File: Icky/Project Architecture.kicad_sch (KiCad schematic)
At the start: 8 parts

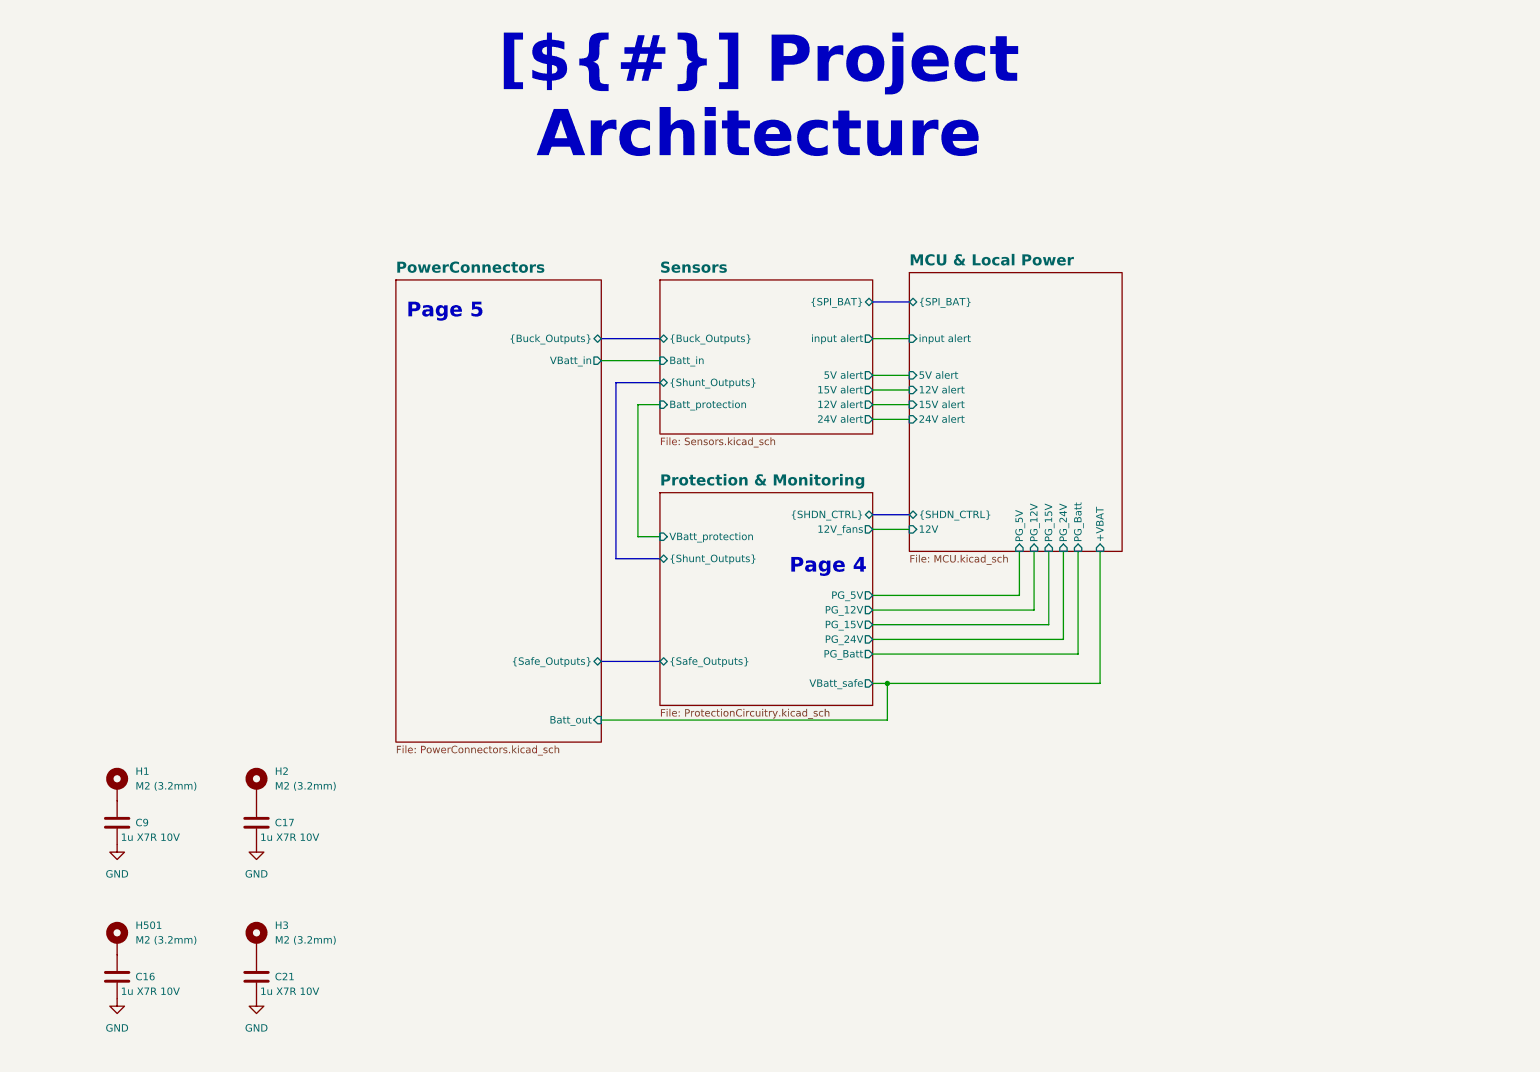
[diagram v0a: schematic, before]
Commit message: ERC passed
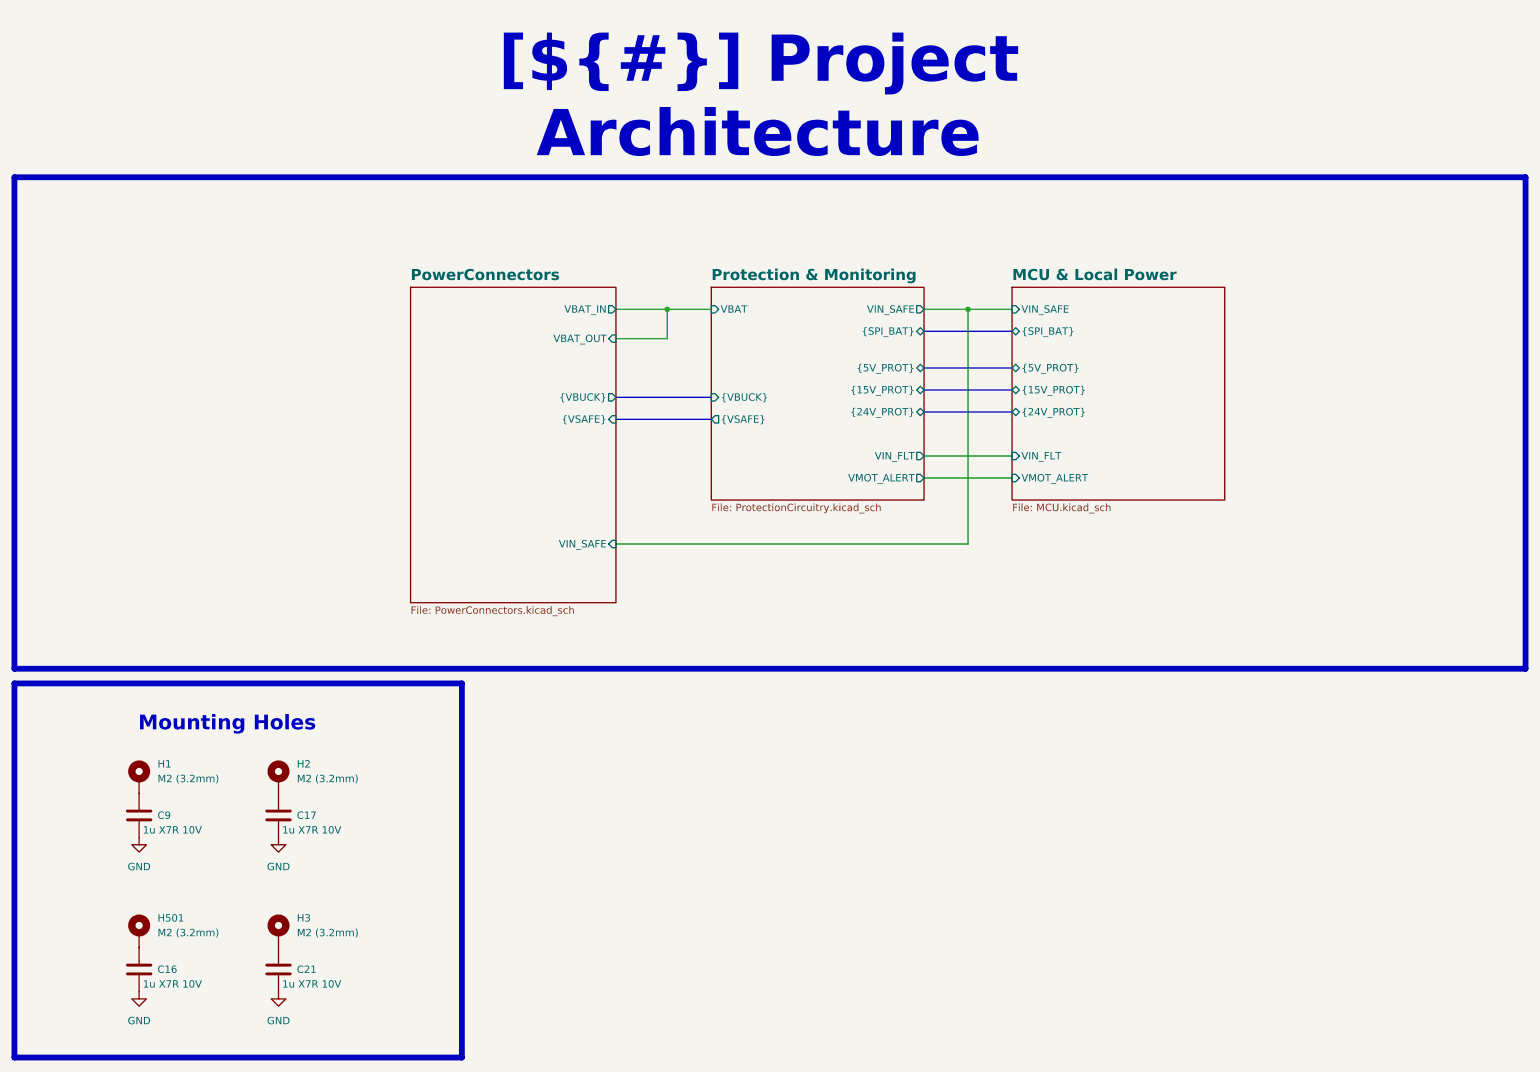
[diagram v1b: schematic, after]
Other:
- removed sheet Sensors
- sheet MCU & Local Power ports: added VIN_FLT, VIN_SAFE, VMOT_ALERT, {15V_PROT}, {24V_PROT}, {5V_PROT}; removed +VBAT, 12V, 12V alert, 15V alert, 24V alert, 5V alert, PG_12V, PG_15V, PG_24V, PG_5V, PG_Batt, input alert, {SHDN_CTRL}
- sheet PowerConnectors ports: added VBAT_IN, VBAT_OUT, VIN_SAFE, {VBUCK}, {VSAFE}; removed Batt_out, VBatt_in, {Buck_Outputs}, {Safe_Outputs}
- sheet Protection & Monitoring ports: added VBAT, VIN_FLT, VIN_SAFE, VMOT_ALERT, {15V_PROT}, {24V_PROT}, {5V_PROT}, {SPI_BAT}, {VBUCK}, {VSAFE}; removed 12V_fans, PG_12V, PG_15V, PG_24V, PG_5V, PG_Batt, VBatt_protection, VBatt_safe, {SHDN_CTRL}, {Safe_Outputs}, {Shunt_Outputs}
- note removed: "Page 4"
- note removed: "Page 5"
- moved on the sheet: C16, C17, C21, C9, H1, H2, H3, H501

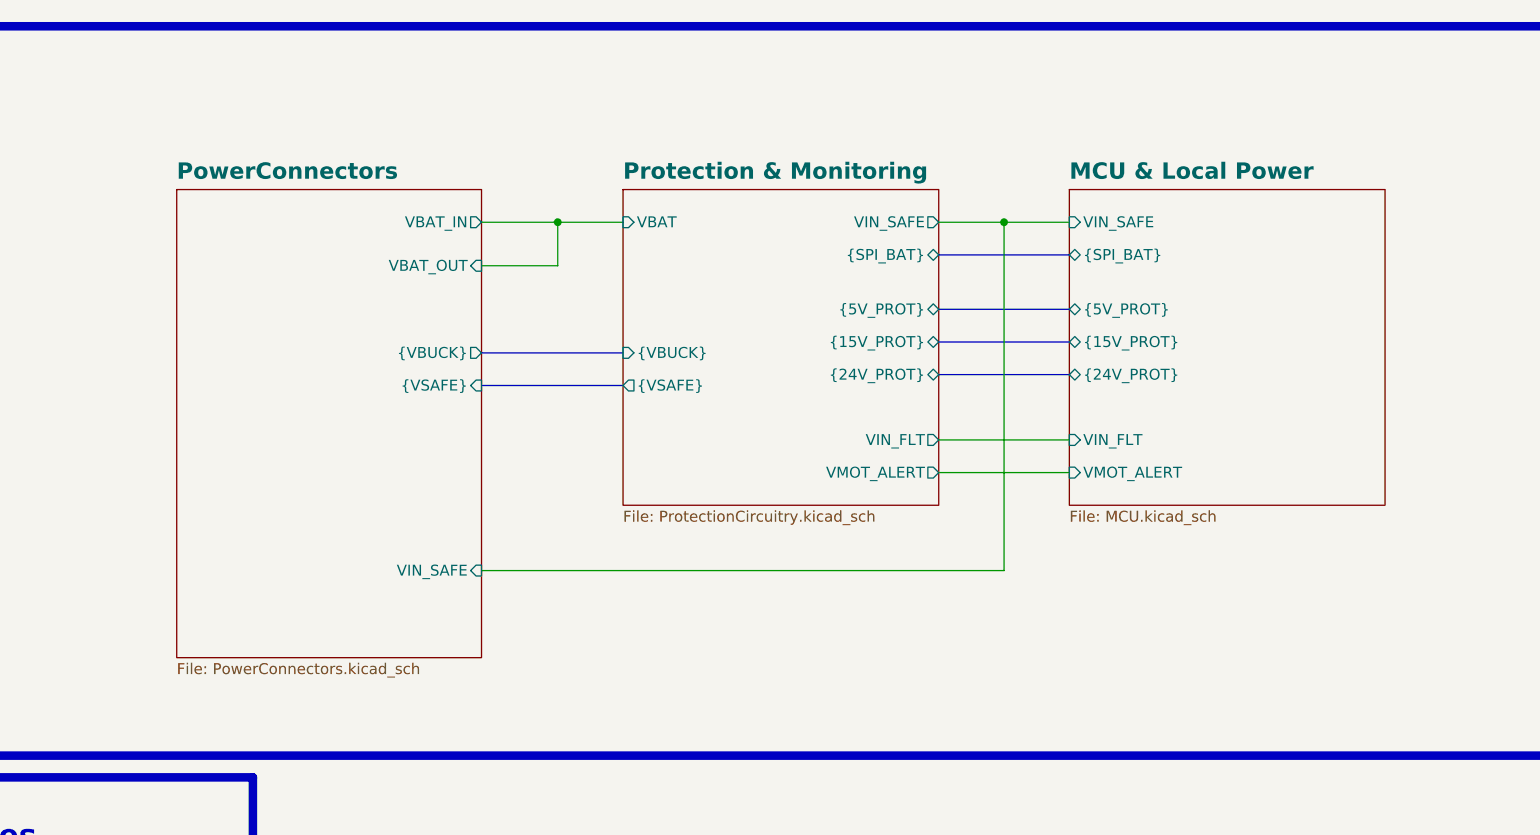
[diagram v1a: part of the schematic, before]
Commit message: ERC passed v2
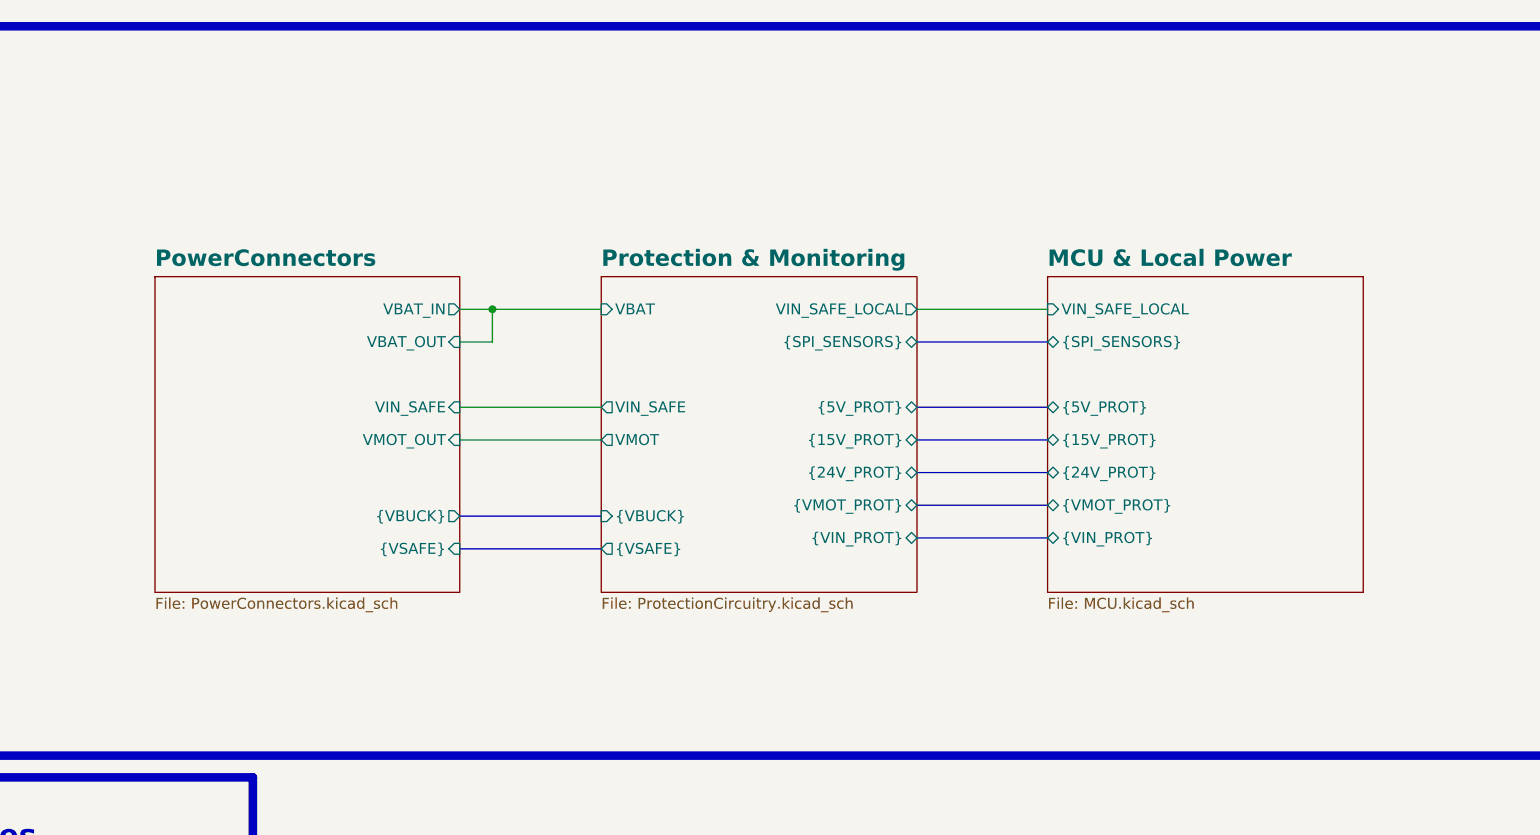
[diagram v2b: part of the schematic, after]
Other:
- sheet MCU & Local Power ports: added VIN_SAFE_LOCAL, {SPI_SENSORS}, {VIN_PROT}, {VMOT_PROT}; removed VIN_FLT, VIN_SAFE, VMOT_ALERT, {SPI_BAT}
- sheet PowerConnectors ports: added VMOT_OUT; removed none
- sheet Protection & Monitoring ports: added VIN_SAFE_LOCAL, VMOT, {SPI_SENSORS}, {VIN_PROT}, {VMOT_PROT}; removed VIN_FLT, VMOT_ALERT, {SPI_BAT}
